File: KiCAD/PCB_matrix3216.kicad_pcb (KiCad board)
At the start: 2 copper layers, 14 parts, among them IC1 NJM7805SDL1-TE1, IC2 NJM2845DL1-33-TE1, J1 Barrel_Jack_Switch, J2 Conn_02x06_Counter_Clockwise, J3 Conn_02x03_Counter_Clockwise, J4 Conn_02x03_Counter_Clockwise, U1 Matrix3216, U2 Matrix3216

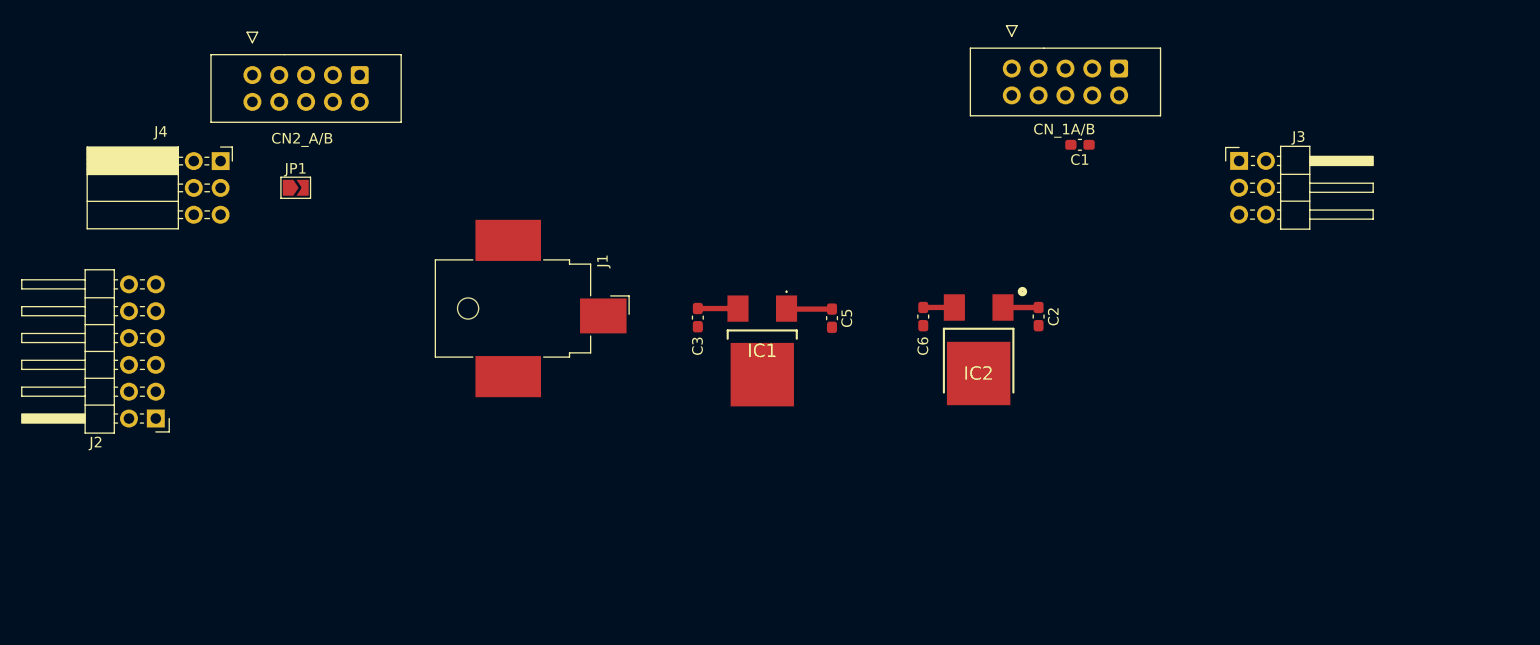
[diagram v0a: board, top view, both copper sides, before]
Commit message: layout
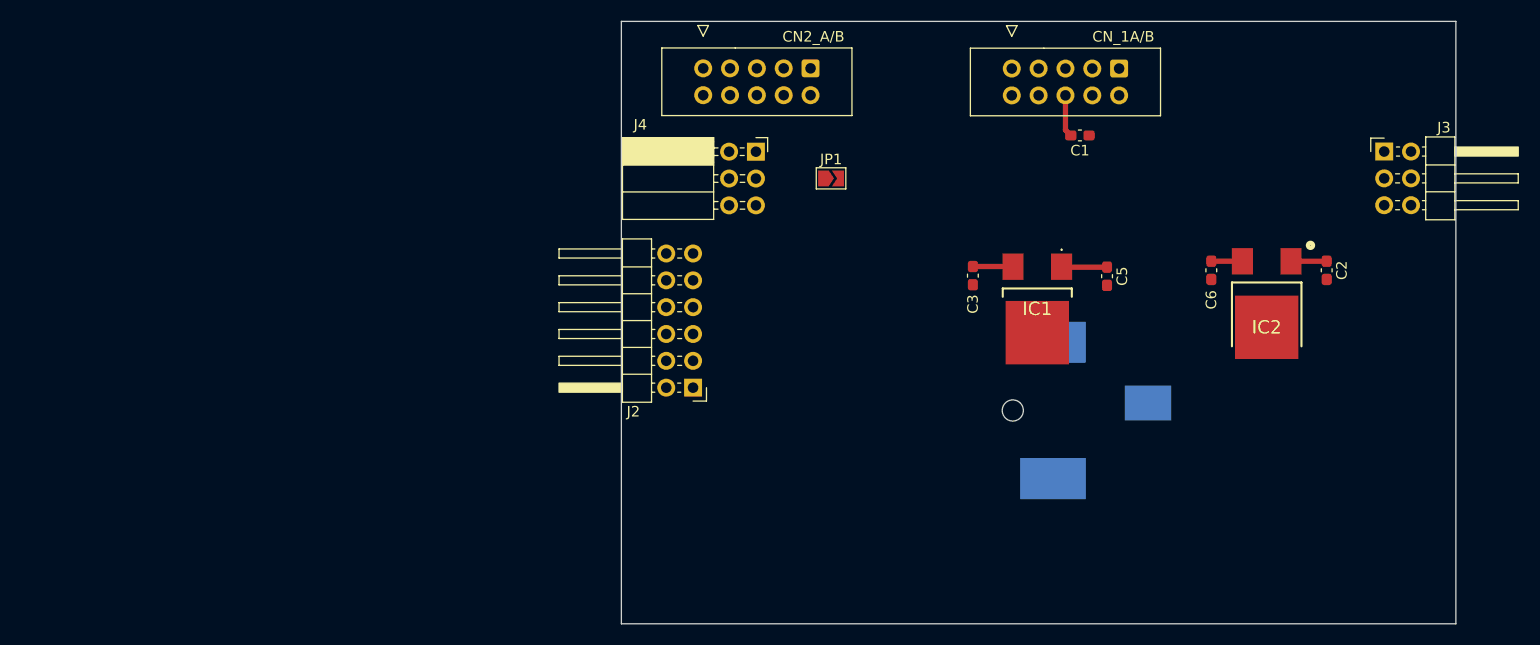
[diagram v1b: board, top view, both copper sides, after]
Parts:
- J1: moved to B.Cu
- moved J1 52.5 mm to (188.7, 97.3), turned to 90 degrees
- moved J2 50.9 mm to (151.4, 95.1)
- moved JP1 50.7 mm to (164.5, 75.3)
- moved J4 50.7 mm to (157.4, 72.8)
- moved U2 42.7 mm to (117.3, 59.8)
- moved C2 27.6 mm to (211.4, 84.0)
- moved C6 27.6 mm to (200.5, 84.0)
- moved IC2 27.6 mm to (205.7, 91.2)
- moved C3 26.3 mm to (177.9, 84.5)
- moved C5 26.3 mm to (190.6, 84.6)
- moved IC1 26.3 mm to (184.0, 87.7)
- moved J3 13.8 mm to (216.9, 72.8)
- moved C1 0.89 mm to (188.1, 71.2)
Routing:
- net +3.3V: track 2.95 -> 6.95 mm
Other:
- board outline added: 79 x 57 mm
